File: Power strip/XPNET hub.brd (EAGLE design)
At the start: 85 x 40 mm, 16 parts, among them X1 MKDSN1,5/4-5,08, X4 MKDSN1,5/4-5,08, X5 MKDSN1,5/4-5,08, X6 MKDSN1,5/4-5,08

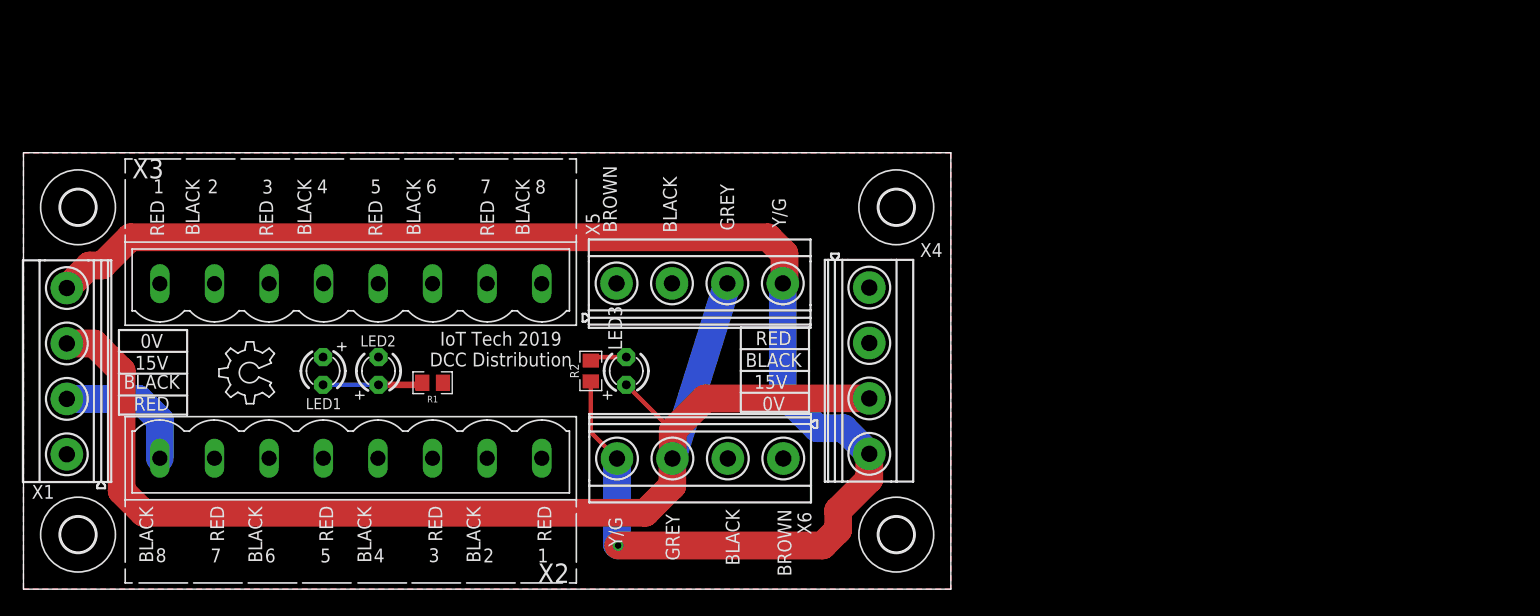
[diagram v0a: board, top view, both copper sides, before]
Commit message: Add files via upload
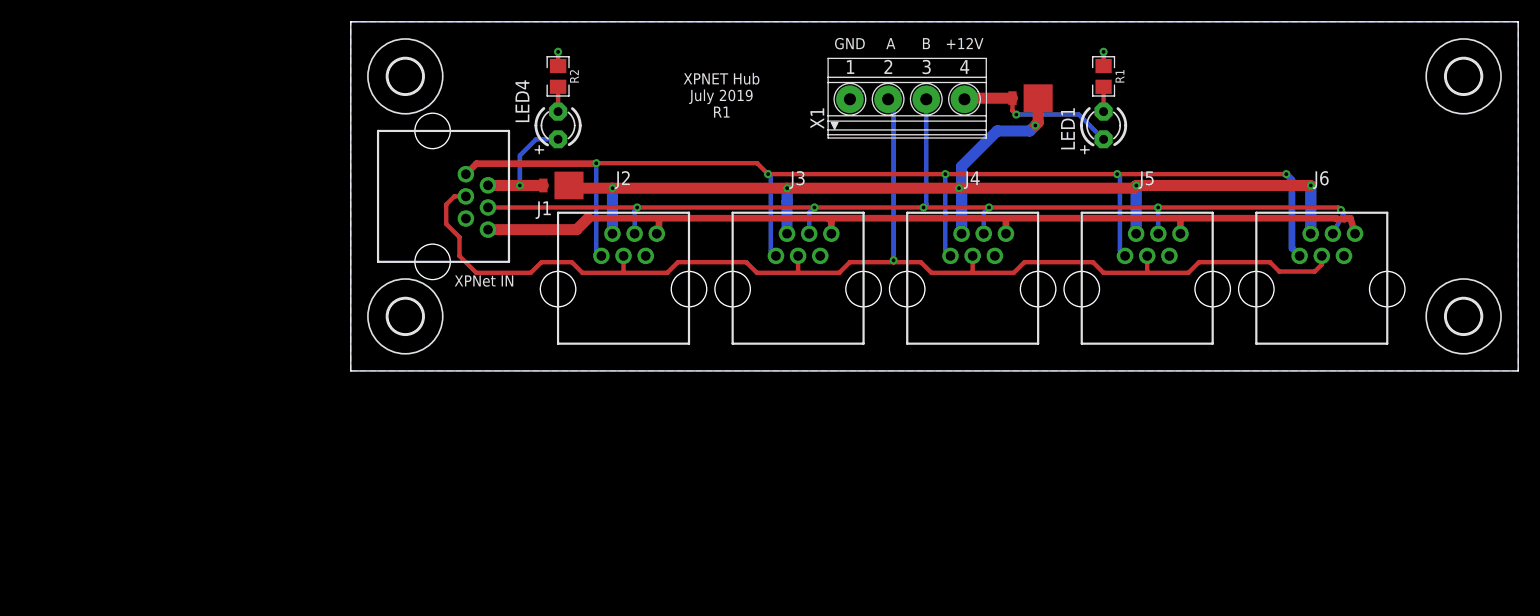
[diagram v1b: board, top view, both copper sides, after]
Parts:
- removed LED2, LED3: Blue, adafruit:LED3MM
- removed LOGO1: OSHW_LOGO_6MILX0200-NT, ohw-logo:OSHW_6X200_NOTEXT
- removed X2, X3: (no value), con-phoenix-500:MSTBV8
- removed X4, X5, X6: MKDSN1,5/4-5,08, con-phoenix-508:MKDSN1,5/4-5,08
- added D1, D2: VISHAY_SCHOTTKY, Ava:DO-220AA
- added J1, J2, J3, J4, J5, J6: RJ11-6SMALL, GJR:RJ11-6-2
- added LED4: Green, adafruit:LED3MM
- LED1: value WHITE -> Green
- X1: value MKDSN1,5/4-5,08 -> 1751264; device con-phoenix-508:MKDSN1,5/4-5,08 -> con-phoenix-350:1751264
- moved H3 128.6 mm to (102.0, 5.00)
- moved X1 81.0 mm to (51.0, 25.0), turned to 0 degrees
- moved LED1 75.0 mm to (69.0, 22.5), turned to 90 degrees
- moved R1 67.6 mm to (69.0, 27.0), turned to 270 degrees
- moved H4 66.8 mm to (102.0, 27.0)
- moved H2 46.6 mm to (5.00, 27.0)
- moved H1 31.6 mm to (5.00, 5.00)
- moved R2 27.2 mm to (19.0, 27.0), turned to 270 degrees
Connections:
- removed net +15V: LED3.A, X1.3, X4.3, X5.3, X6.3
- removed net DCC1: LED1.A, LED2.K, X1.1, X2.1, X2.3, X2.5, X2.7, X3.1, X3.3, X3.5, X3.7, X4.1, X5.1, X6.1
- removed net DCC2: R1.1, X1.2, X2.2, X2.4, X2.6, X2.8, X3.2, X3.4, X3.6, X3.8, X4.2, X5.2, X6.2
- removed net N$32: LED1.K, LED2.A, R1.2
- new net +12V: D1.CATHODE, D2.CATHODE, J2.5, J3.5, J4.5, J5.5, J6.5
- new net +21V1: D2.ANODE, LED1.A, X1.4
- new net A: J1.4, J2.4, J3.4, J4.4, J5.4, J6.4, X1.2
- new net B: J1.3, J2.3, J3.3, J4.3, J5.3, J6.3, X1.3
- new net CMD_ACK: J1.6, J2.6, J3.6, J4.6, J5.6, J6.6
- new net GND_RTN: J1.1, J2.1, J3.1, J4.1, J5.1, J6.1
- new net N$19: LED4.K, R2.2
- new net N$3: LED1.K, R1.2
- net GND: now also J1.2, J2.2, J3.2, J4.2, J5.2, J6.2, R1.1, X1.1; no longer X1.4, X4.4, X5.4, X6.4
- net N$1: now also D1.ANODE, J1.5, LED4.A; no longer LED3.K, R2.2
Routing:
- net GND: track 136.4 -> 2.60 mm, vias 1 -> 2
- net +15V: track 116.5 -> 0.00 mm
- net CMD_ACK: track 0.00 -> 116.2 mm, vias 0 -> 5
- net A: track 0.00 -> 113.4 mm, vias 0 -> 1
- net +12V: track 0.00 -> 106.8 mm, vias 0 -> 6
- net B: track 0.00 -> 100.9 mm, vias 0 -> 6
- net GND_RTN: track 0.00 -> 87.0 mm
- net +21V1: track 0.00 -> 15.0 mm, vias 0 -> 1
- net DCC2: track 12.8 -> 0.00 mm
- net N$32: track 9.14 -> 0.00 mm
- net N$1: track 3.42 -> 11.9 mm, vias 0 -> 1
- net N$3: track 0.00 -> 2.28 mm
- net N$19: track 0.00 -> 2.28 mm
- added copper zone on layer 16, net GND
- removed copper zone on layer 16, net DCC1
- removed copper zone on layer 1, net DCC2
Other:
- board size 85 x 40 mm -> 107 x 32 mm
- board text added: "+12V"
- board text added: "A"
- board text added: "B"
- board text added: "GND"
- board text added: "XPNET Hub July 2019 R1"
- board text added: "XPNet IN"
- board text removed: "0V"
- board text removed: "15V"
- board text removed: "BLACK"
- board text removed: "BROWN"
- board text removed: "GREY"
- board text removed: "IoT Tech 2019 DCC Distribution"
- board text removed: "RED"
- board text removed: "Y/G"
